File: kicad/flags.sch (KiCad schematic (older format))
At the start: 3 parts, among them U48 74LS173

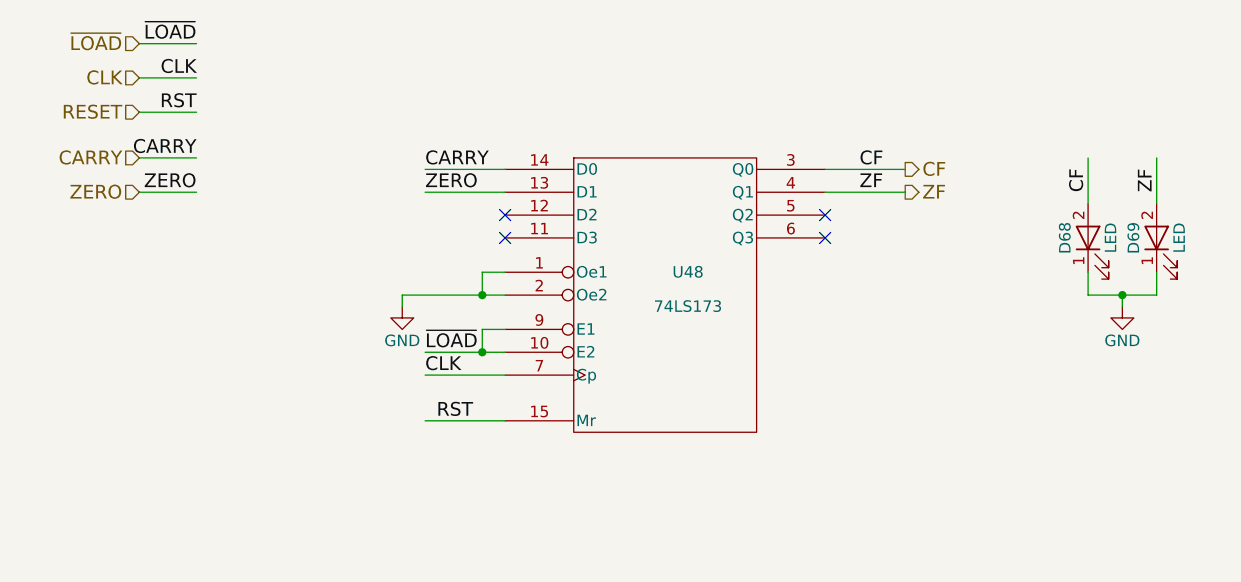
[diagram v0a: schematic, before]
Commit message: Update to current kicad libraries
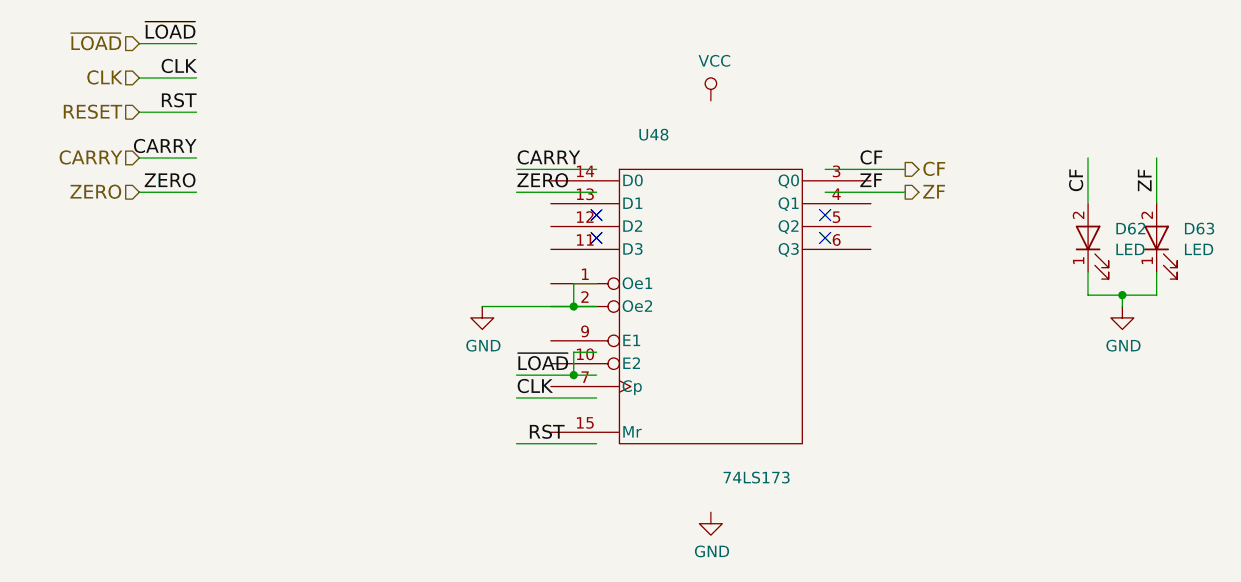
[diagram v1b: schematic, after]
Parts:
- removed D68, D69: LED, symbol LED
- removed U48: 74LS173, symbol 74LS173
- added D62, D63: LED, symbol Device:LED
- added U48: 74LS173, symbol 74xx:74LS173
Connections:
- net labels added: VCC
- wire segments 27 -> 26
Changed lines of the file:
@@
-EESchema Schematic File Version 2
-LIBS:power
-LIBS:device
-LIBS:transistors
-LIBS:conn
-LIBS:linear
-LIBS:regul
-LIBS:74xx
-LIBS:cmos4000
-LIBS:adc-dac
-LIBS:memory
-LIBS:xilinx
-LIBS:microcontrollers
-LIBS:dsp
-LIBS:microchip
-LIBS:analog_switches
-LIBS:motorola
-LIBS:texas
-LIBS:intel
-LIBS:audio
-LIBS:interface
-LIBS:digital-audio
-LIBS:philips
-LIBS:display
-LIBS:cypress
-LIBS:siliconi
-LIBS:opto
-LIBS:atmel
-LIBS:contrib
-LIBS:valves
-LIBS:switches
-LIBS:74xxx
-LIBS:28c16
-LIBS:sap-be-cache
-EELAYER 24 0
+EESchema Schematic File Version 4
+EELAYER 30 0
 EELAYER END
 $Descr A4 11693 8268
 encoding utf-8
-Sheet 12 12
+Sheet 12 13
 Title "Simple As Possible computer by Ben Eater"
 Date "2017-05-10"
@@
 Text HLabel 4650 1600 2    60   Output ~ 0
 ZF
-$Comp
-L 74LS173 U48
-U 1 1 5AD47646
-P 3600 2050
-F 0 "U48" H 3700 2150 50  0000 C CNN
-F 1 "74LS173" H 3700 2000 50  0000 C CNN
-F 2 "" H 3600 2050 50  0000 C CNN
-F 3 "" H 3600 2050 50  0000 C CNN
-	1    3600 2050
-	1    0    0    -1
-$EndComp
 Text Label 1550 950  2    60   ~ 0
 ~LOAD
-Text Label 2550 2300 0    60   ~ 0
+Text Label 2950 2400 0    60   ~ 0
 ~LOAD
-$Comp
-L GND #PWR090
-U 1 1 5AD4767C
-P 2450 2100
-F 0 "#PWR090" H 2450 1850 50  0001 C CNN
-F 1 "GND" H 2450 1950 50  0000 C CNN
-F 2 "" H 2450 2100 50  0000 C CNN
-F 3 "" H 2450 2100 50  0000 C CNN
-	1    2450 2100
-	1    0    0    -1
-$EndComp
-Text Label 2550 1500 0    60   ~ 0
+Text Label 2950 1500 0    60   ~ 0
 CARRY
-Text Label 2550 1600 0    60   ~ 0
+Text Label 2950 1600 0    60   ~ 0
 ZERO
 Text Label 1550 1450 2    60   ~ 0
@@
 Text Label 1550 1250 2    60   ~ 0
 RST
-Text Label 2600 2600 0    60   ~ 0
+Text Label 3000 2700 0    60   ~ 0
 RST
 Wire Wire Line
 	1550 950  1300 950
 Wire Wire Line
-	2550 2300 2800 2300
+	2950 2400 3200 2400
 Wire Wire Line
-	2800 2300 2900 2300
+	3200 2400 3300 2400
 Wire Wire Line
-	2800 2300 2800 2200
+	3200 2400 3200 2300
 Wire Wire Line
-	2800 2200 2900 2200
-Connection ~ 2800 2300
+	3200 2300 3300 2300
+Connection ~ 3200 2400
 Wire Wire Line
-	2900 2050 2800 2050
+	3300 2100 3200 2100
 Wire Wire Line
-	2800 2050 2450 2050
+	3300 2000 3200 2000
 Wire Wire Line
-	2450 2050 2450 2100
+	3200 2000 3200 2100
+Connection ~ 3200 2100
 Wire Wire Line
-	2900 1950 2800 1950
+	2950 1500 3300 1500
 Wire Wire Line
-	2800 1950 2800 2050
-Connection ~ 2800 2050
-Wire Wire Line
-	2550 1500 2900 1500
-Wire Wire Line
-	2550 1600 2900 1600
+	2950 1600 3300 1600
 Wire Wire Line
 	1550 1450 1300 1450
@@
 	1550 1100 1300 1100
 Wire Wire Line
-	2550 2600 2900 2600
+	2950 2700 3300 2700
 Wire Wire Line
-	2550 2400 2900 2400
-Text Label 2550 2400 0    60   ~ 0
+	2950 2500 3300 2500
+Text Label 2950 2500 0    60   ~ 0
 CLK
 Text Label 4450 1500 0    60   ~ 0
@@
 NoConn ~ 4300 1700
 NoConn ~ 4300 1800
-NoConn ~ 2900 1700
-NoConn ~ 2900 1800
-$Comp
-L LED D68
-U 1 1 5AD4AD3C
-P 5450 1800
-F 0 "D68" H 5450 1900 50  0000 C CNN
-F 1 "LED" H 5450 1700 50  0000 C CNN
-F 2 "" H 5450 1800 50  0000 C CNN
-F 3 "" H 5450 1800 50  0000 C CNN
-	1    5450 1800
-	0    -1   -1   0
-$EndComp
-$Comp
-L LED D69
-U 1 1 5AD4AD4E
-P 5750 1800
-F 0 "D69" H 5750 1900 50  0000 C CNN
-F 1 "LED" H 5750 1700 50  0000 C CNN
-F 2 "" H 5750 1800 50  0000 C CNN
-F 3 "" H 5750 1800 50  0000 C CNN
-	1    5750 1800
-	0    -1   -1   0
-$EndComp
-$Comp
-L GND #PWR091
-U 1 1 5AD4AD59
-P 5600 2100
-F 0 "#PWR091" H 5600 1850 50  0001 C CNN
-F 1 "GND" H 5600 1950 50  0000 C CNN
-F 2 "" H 5600 2100 50  0000 C CNN
-F 3 "" H 5600 2100 50  0000 C CNN
-	1    5600 2100
-	1    0    0    -1
-$EndComp
+NoConn ~ 3300 1700
+NoConn ~ 3300 1800
 Wire Wire Line
 	5600 2100 5600 2050
@@
 Text Label 5750 1600 1    60   ~ 0
 ZF
+$Comp
+L power:GND #PWR0156
+U 1 1 5EA8388C
+P 2800 2100
+F 0 "#PWR0156" H 2800 1850 50  0001 C CNN
+F 1 "GND" H 2805 1927 50  0000 C CNN
+F 2 "" H 2800 2100 50  0001 C CNN
+F 3 "" H 2800 2100 50  0001 C CNN
+	1    2800 2100
+	1    0    0    -1
+$EndComp
+Wire Wire Line
+	2800 2100 3200 2100
+$Comp
+L power:GND #PWR0159
+U 1 1 5EA8545C
+P 5600 2100
+F 0 "#PWR0159" H 5600 1850 50  0001 C CNN
+F 1 "GND" H 5605 1927 50  0000 C CNN
+F 2 "" H 5600 2100 50  0001 C CNN
+F 3 "" H 5600 2100 50  0001 C CNN
+	1    5600 2100
+	1    0    0    -1
+$EndComp
+$Comp
+L Device:LED D62
+U 1 1 5EA85B93
+P 5450 1800
+F 0 "D62" V 5489 1683 50  0000 R CNN
+F 1 "LED" V 5398 1683 50  0000 R CNN
+F 2 "" H 5450 1800 50  0001 C CNN
+F 3 "~" H 5450 1800 50  0001 C CNN
+	1    5450 1800
+	0    -1   -1   0
+$EndComp
+$Comp
+L Device:LED D63
+U 1 1 5EA8646D
+P 5750 1800
+F 0 "D63" V 5789 1683 50  0000 R CNN
+F 1 "LED" V 5698 1683 50  0000 R CNN
+F 2 "" H 5750 1800 50  0001 C CNN
+F 3 "~" H 5750 1800 50  0001 C CNN
+	1    5750 1800
+	0    -1   -1   0
+$EndComp
+$Comp
+L 74xx:74LS173 U48
+U 1 1 5EA87D23
+P 3800 2100
+F 0 "U48" H 3550 2850 50  0000 C CNN
+F 1 "74LS173" H 4000 1350 50  0000 C CNN
+F 2 "" H 3800 2100 50  0001 C CNN
+F 3 "http://www.ti.com/lit/gpn/sn74LS173" H 3800 2100 50  0001 C CNN
+	1    3800 2100
+	1    0    0    -1
+$EndComp
+$Comp
+L power:GND #PWR0158
+U 1 1 5EA8EB64
+P 3800 3000
+F 0 "#PWR0158" H 3800 2750 50  0001 C CNN
+F 1 "GND" H 3805 2827 50  0000 C CNN
+F 2 "" H 3800 3000 50  0001 C CNN
+F 3 "" H 3800 3000 50  0001 C CNN
+	1    3800 3000
+	1    0    0    -1
+$EndComp
+$Comp
+L power:VCC #PWR0157
+U 1 1 5EA8F117
+P 3800 1200
+F 0 "#PWR0157" H 3800 1050 50  0001 C CNN
+F 1 "VCC" H 3817 1373 50  0000 C CNN
+F 2 "" H 3800 1200 50  0001 C CNN
+F 3 "" H 3800 1200 50  0001 C CNN
+	1    3800 1200
+	1    0    0    -1
+$EndComp
 $EndSCHEMATC
